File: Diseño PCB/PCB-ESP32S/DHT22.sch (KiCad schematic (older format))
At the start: 2 parts

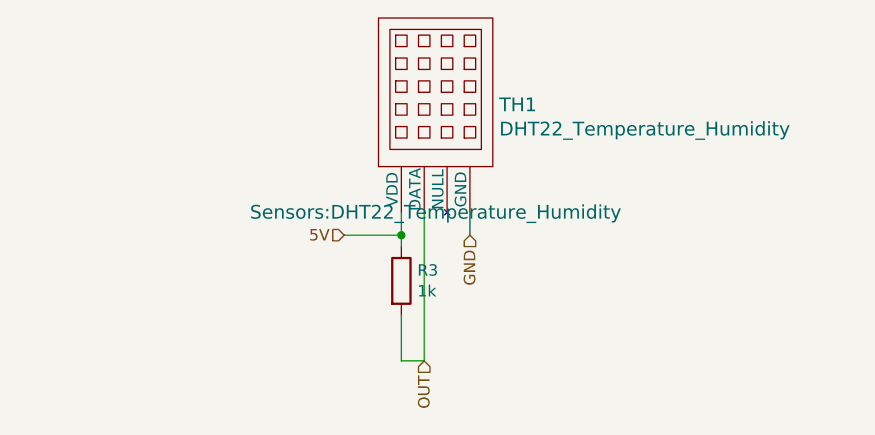
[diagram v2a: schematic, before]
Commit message: pcv v2
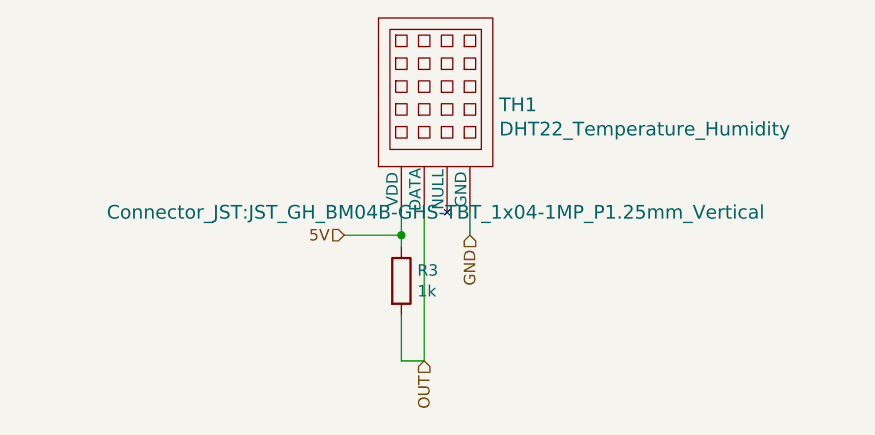
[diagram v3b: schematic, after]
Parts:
- TH1: footprint Sensors:DHT22_Temperature_Humidity -> Connector_JST:JST_GH_BM04B-GHS-TBT_1x04-1MP_P1.25mm_Vertical
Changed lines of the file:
@@
 F 0 "TH1" H 2778 2820 60  0000 L CNN
 F 1 "DHT22_Temperature_Humidity" H 2778 2714 60  0000 L CNN
-F 2 "Sensors:DHT22_Temperature_Humidity" H 2500 2350 60  0000 C CNN
+F 2 "Connector_JST:JST_GH_BM04B-GHS-TBT_1x04-1MP_P1.25mm_Vertical" H 2500 2350 60  0000 C CNN
 F 3 "" H 2500 2350 60  0000 C CNN
 	1    2500 2350

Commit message: mejoras pcb1
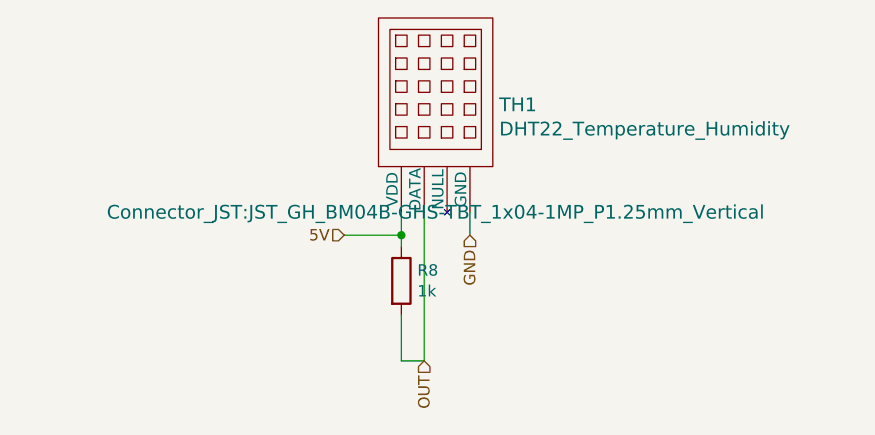
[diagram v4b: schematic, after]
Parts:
- renumbered R3 to R8
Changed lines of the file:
@@
 P 2350 2650
 AR Path="/61A00339" Ref="R?"  Part="1"
-AR Path="/61A137FE/61A00339" Ref="R3"  Part="1"
-F 0 "R3" H 2420 2696 50  0000 L CNN
+AR Path="/61A137FE/61A00339" Ref="R8"  Part="1"
+F 0 "R8" H 2420 2696 50  0000 L CNN
 F 1 "1k" H 2420 2605 50  0000 L CNN
 F 2 "Resistor_SMD:R_0805_2012Metric_Pad1.20x1.40mm_HandSolder" V 2280 2650 50  0001 C CNN
